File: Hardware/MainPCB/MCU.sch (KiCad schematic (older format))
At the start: 22 parts, among them J2 Conn_01x11, J3 UART, U4 ESP32-WROOM-32D, U5 TPS22919, U6 TPS22919, U7 TPS22919

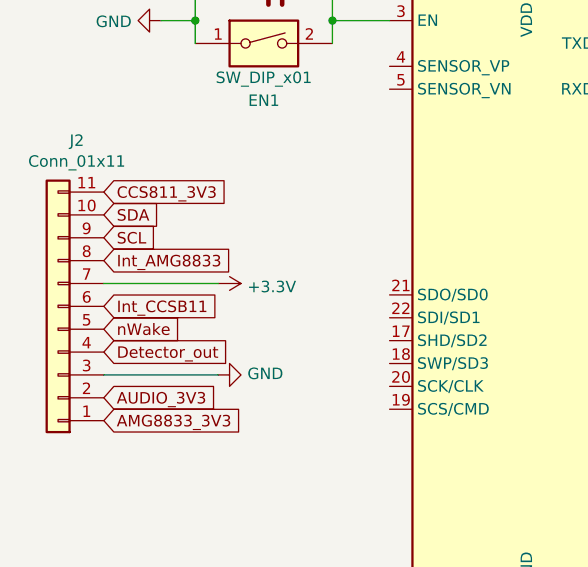
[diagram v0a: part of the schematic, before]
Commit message: Finished MainPCB + generated gerber files + aanpassingen BOM
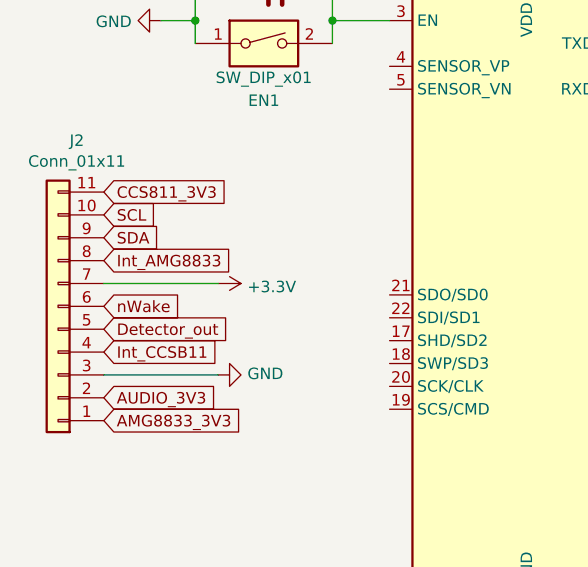
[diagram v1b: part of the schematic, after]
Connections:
- net Detector_out: now also J2.5 (Pin_5); no longer J2.4 (Pin_4)
- net Int_CCSB11: now also J2.4 (Pin_4); no longer J2.6 (Pin_6)
- net SCL: now also J2.10 (Pin_10); no longer J2.9 (Pin_9)
- net SDA: now also J2.9 (Pin_9); no longer J2.10 (Pin_10)
- net nWake: now also J2.6 (Pin_6); no longer J2.5 (Pin_5)
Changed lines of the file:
@@
 Text GLabel 3800 4550 2    50   Input ~ 0
 SDA
+Text GLabel 1150 4100 2    50   Input ~ 0
+SDA
 Text GLabel 1150 4000 2    50   Input ~ 0
-SDA
-Text GLabel 1150 4100 2    50   Input ~ 0
 SCL
 Wire Wire Line
@@
 Text GLabel 1150 4200 2    50   Input ~ 0
 Int_AMG8833
+Text GLabel 1150 4600 2    50   Input ~ 0
+Int_CCSB11
 Text GLabel 1150 4400 2    50   Input ~ 0
-Int_CCSB11
+nWake
 Text GLabel 1150 4500 2    50   Input ~ 0
-nWake
-Text GLabel 1150 4600 2    50   Input ~ 0
 Detector_out
 Text GLabel 3600 4950 2    50   Input ~ 0
